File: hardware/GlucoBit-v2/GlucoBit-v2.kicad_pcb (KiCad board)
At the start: 4 copper layers, 55 x 30.4 mm, 43 parts, among them J1 USB-C-P16, J2 B2B-PH-K-S, J3 Conn_01x02_Socket, J6 B2B-PH-K-S, SW1 RESET, SW2 BOOT, U1 ESP32-S3-WROOM-1-N8, U2 BQ24040DSQR, U3 TLV75801PDBV, U4 USBLC6-2SC6, U5 MAX98357AETE+T, U6 08JQ-BT

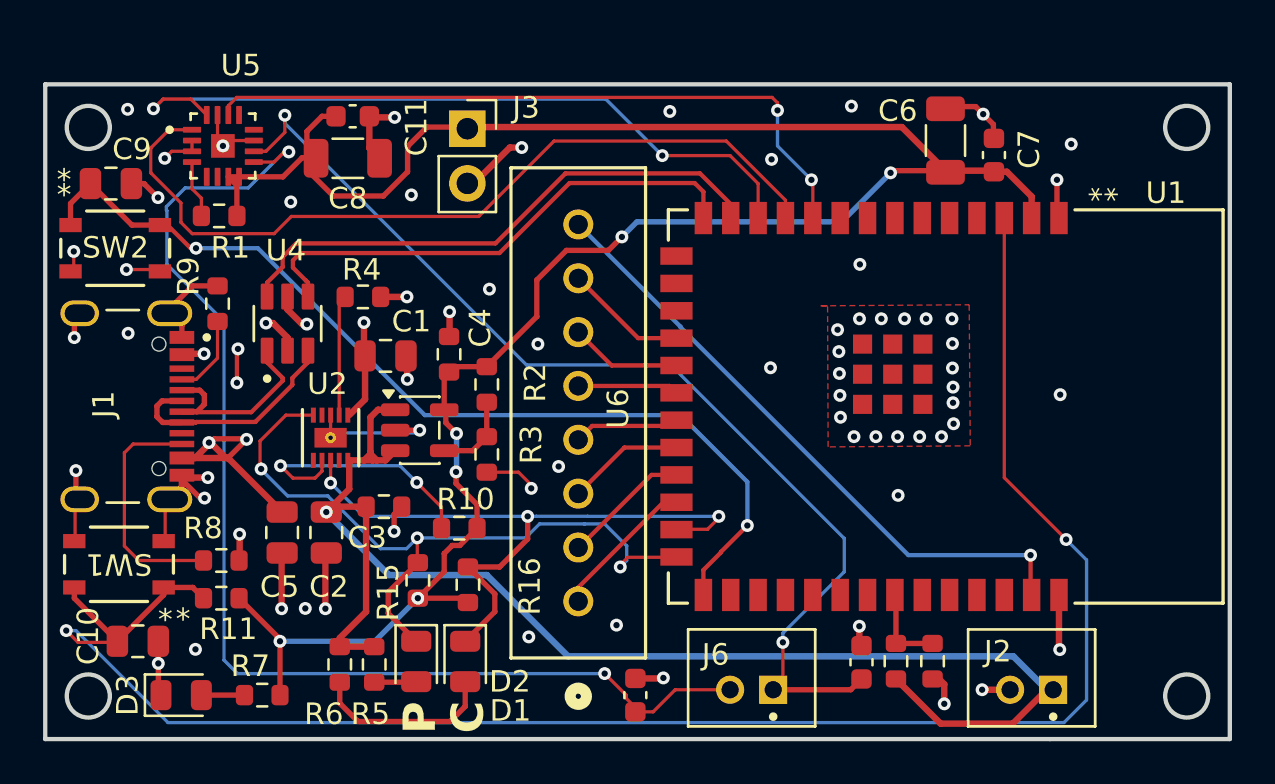
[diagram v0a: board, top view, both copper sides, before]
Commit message: Generated STEP files
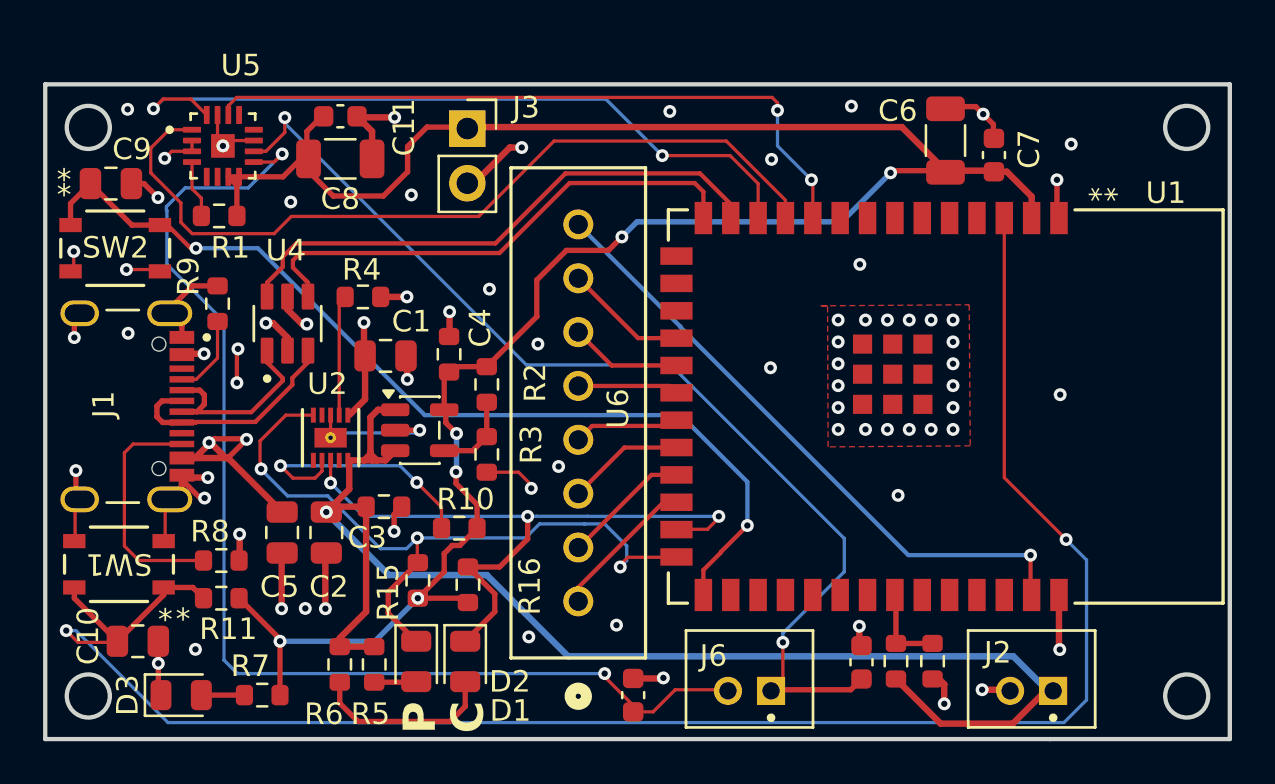
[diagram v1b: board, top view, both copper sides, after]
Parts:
- moved C11 0.57 mm to (130.3, 75.1)
- moved C8 0.35 mm to (130.3, 77.1)
- moved J6 0.11 mm to (149.3, 101.2)
- moved C12 0.10 mm to (143.9, 102.0)
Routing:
- net +3V3: track 105.3 -> 103.8 mm
- net GND: track 68.7 -> 69.5 mm
- net Net-(U5-OUTP): track 55.8 -> 55.2 mm
